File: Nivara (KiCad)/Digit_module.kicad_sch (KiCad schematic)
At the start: 8 parts

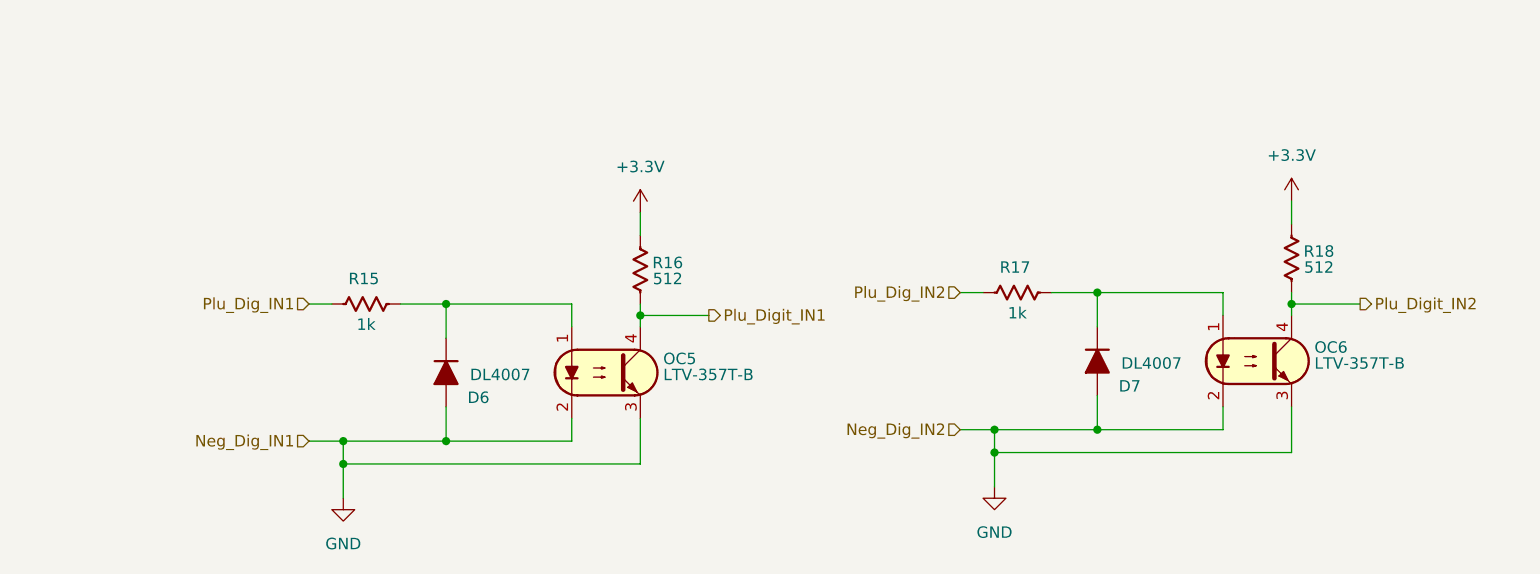
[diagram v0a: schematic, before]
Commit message: Add files via upload
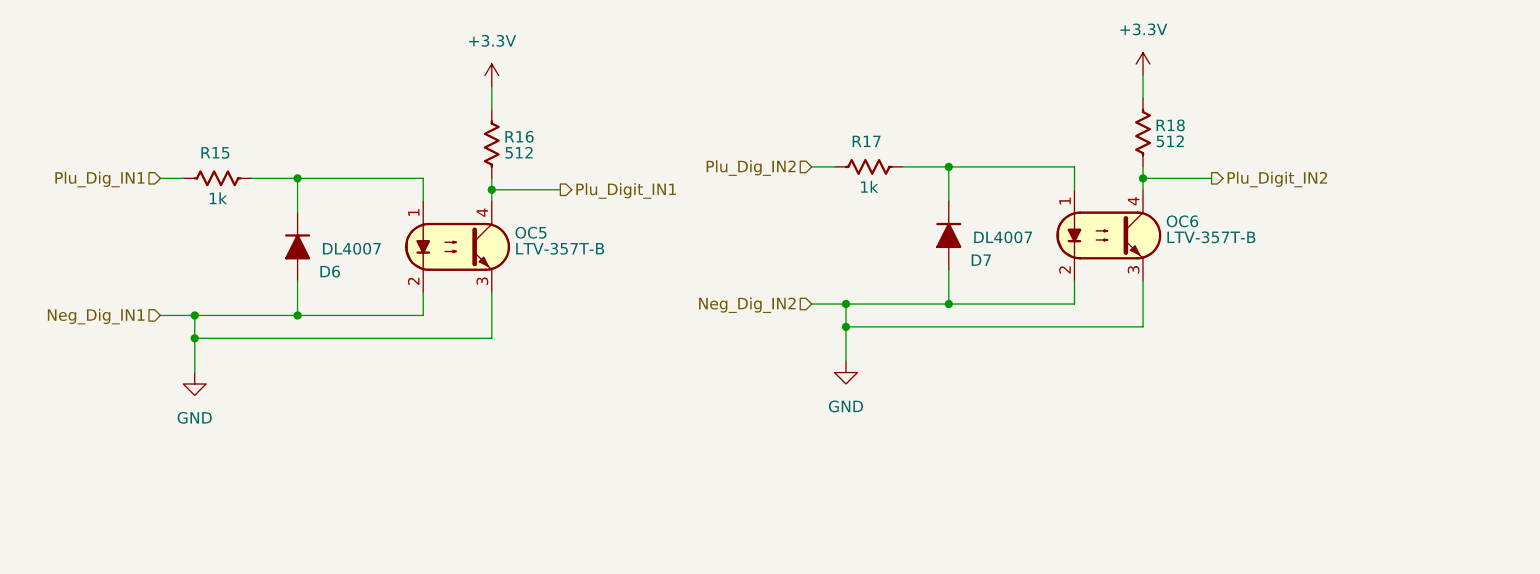
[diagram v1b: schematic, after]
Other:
- moved on the sheet: D6, D7, OC5, OC6, R15, R16, R17, R18
